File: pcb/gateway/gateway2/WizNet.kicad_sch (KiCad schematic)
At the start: 36 parts, among them J2 RJ45_Kycon_G7LX-A88S7-BP-GY, U2 W6300-Q, Y2 25MHz

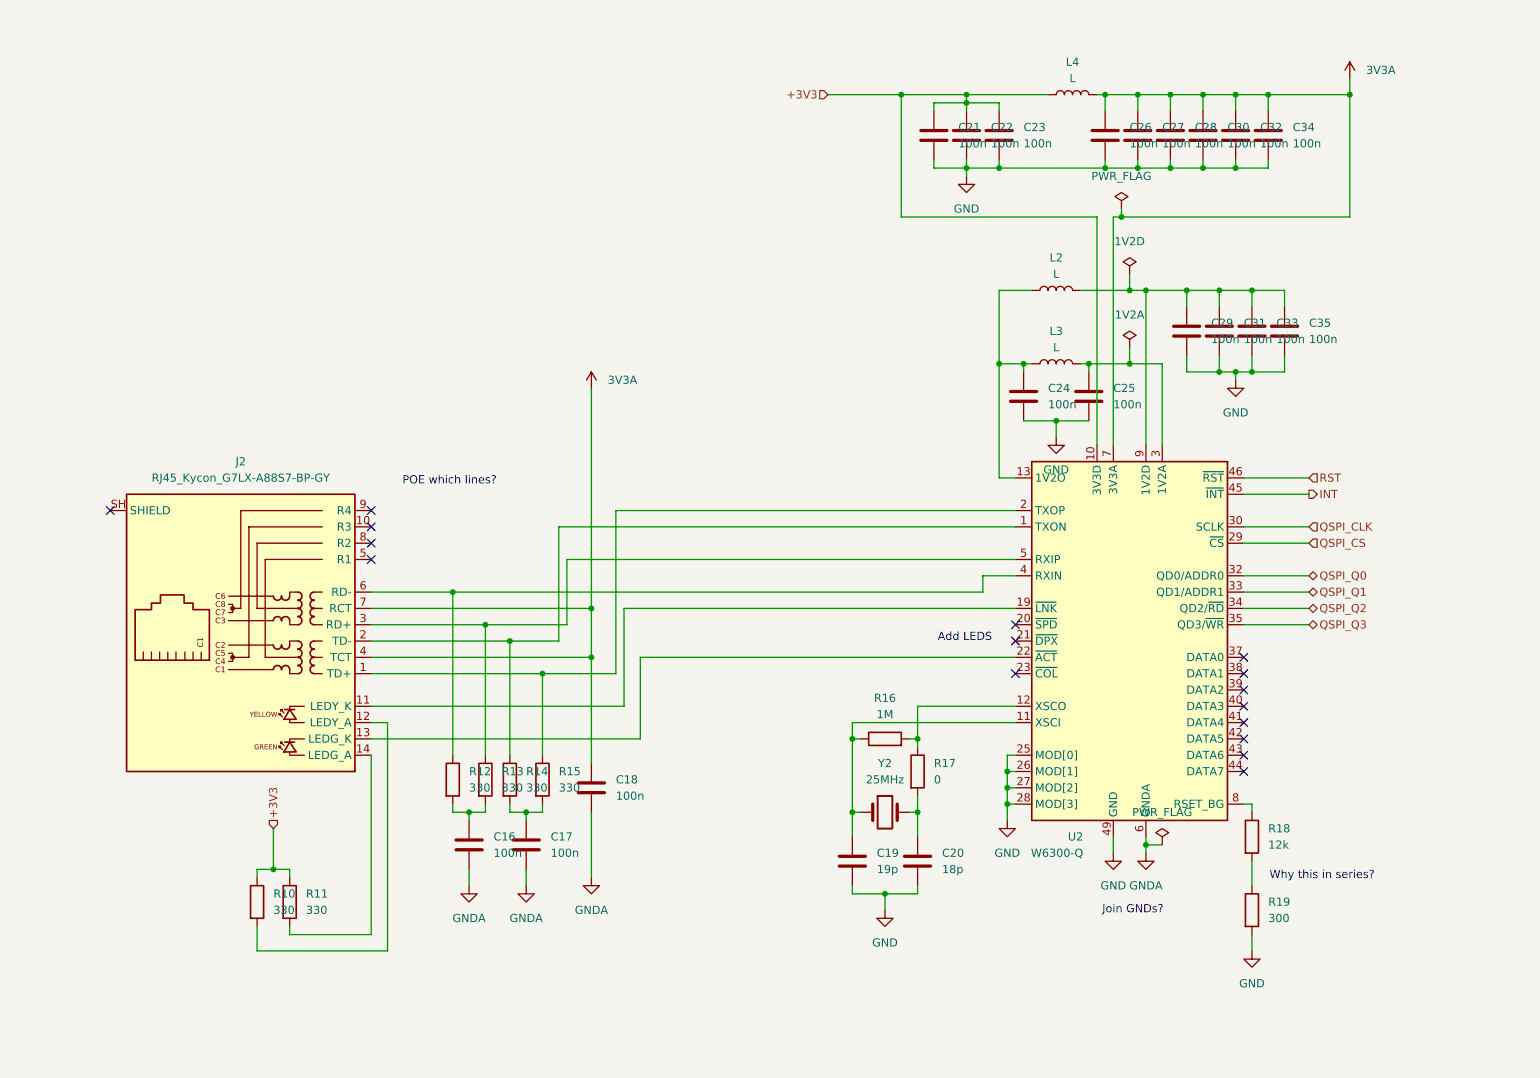
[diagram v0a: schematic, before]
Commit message: Starting to look at routing.
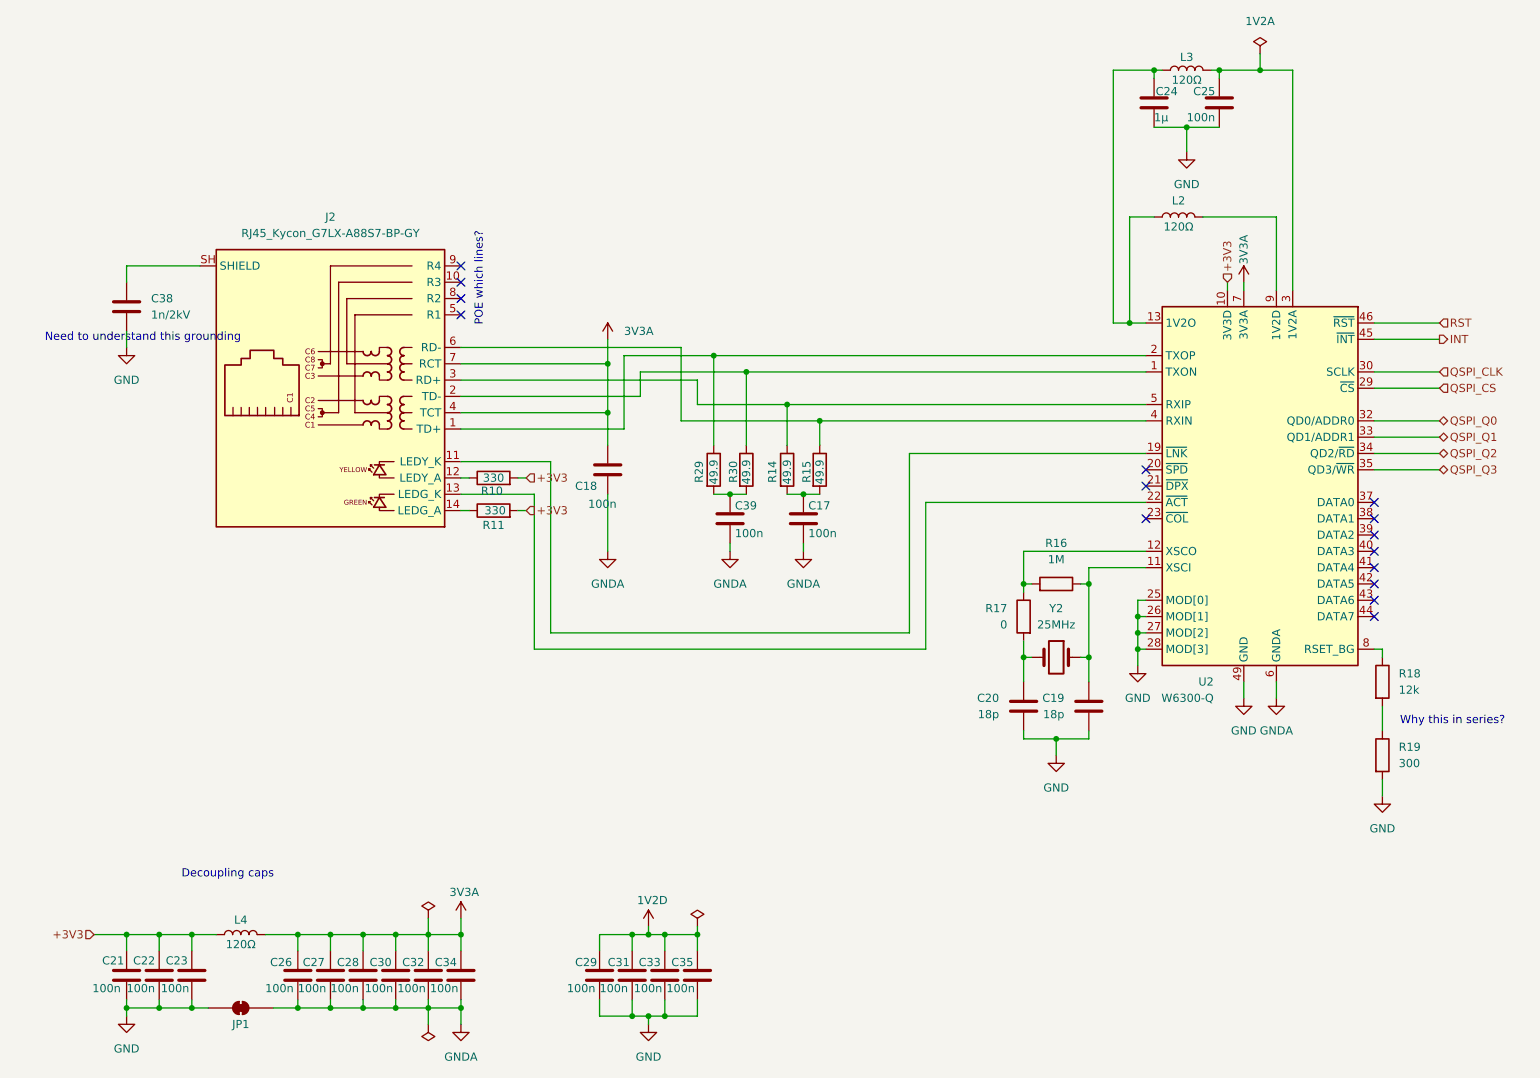
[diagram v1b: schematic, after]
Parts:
- removed C16: 100n, Capacitor_SMD:C_0603_1608Metric, symbol Device:C
- removed R12, R13: 330, Resistor_SMD:R_0603_1608Metric, symbol Device:R
- added C38: 1n/2kV, Capacitor_SMD:C_0603_1608Metric, symbol Device:C
- added C39: 100n, Capacitor_SMD:C_0603_1608Metric, symbol Device:C
- added JP1: SolderJumper_2_Bridged, symbol Jumper:SolderJumper_2_Bridged
- added R29, R30: 49.9, Resistor_SMD:R_0603_1608Metric, symbol Device:R
- C19: value 19p -> 18p
- C24: value 100n -> 1µ
- L2, L3, L4: value L -> 120Ω; MPN (none) -> MPZ1608S121ATDH5
- R14, R15: value 330 -> 49.9
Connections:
- net 3V3D: now also R10.2, R11.2; no longer R10.1, R11.1
- net GND: now also C38.1, JP1.1 (A); no longer C26.1, C27.1, C28.1, C30.1, C32.1, C34.1
- net GNDA: now also C26.1, C27.1, C28.1, C30.1, C32.1, C34.1, C39.1, JP1.2 (B)
- net at J2.6 (RD-), U2.4 (RXIN): now also R15.1
- net at J2.1 (TD+), U2.2 (TXOP): now also R29.1; no longer R15.1
- net at J2.2 (TD-), U2.1 (TXON): now also R30.1; no longer R14.1
- net at J2.3 (RD+), U2.5 (RXIP): now also R14.1
- net at J2.12 (LEDY_A): now also R10.1; no longer R10.2
- net at J2.14 (LEDG_A): now also R11.1; no longer R11.2
- net at J2.SH (SHIELD): now also C38.2
- new net: C39.2, R29.2, R30.2
- no-connect marks 16 -> 15
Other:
- note added: "Decoupling caps"
- note added: "Need to understand this grounding"
- note removed: "Add LEDS"
- note removed: "Join GNDs?"
- moved on the sheet: C17, C18, C19, C20, C21, C22, C23, C24, C25, C26, C27, C28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
